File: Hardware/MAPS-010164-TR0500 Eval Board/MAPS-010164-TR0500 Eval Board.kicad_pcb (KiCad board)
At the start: 2 copper layers, 48.5 x 38.8 mm, 23 parts, among them IC1 MAPS-010164-TR0500, J1 Conn_Coaxial, J2 Conn_Coaxial, J3 Conn_02x02_Top_Bottom, J4 Conn_02x02_Top_Bottom, J5 Conn_02x04_Top_Bottom, J6 Conn_Coaxial, J7 Conn_Coaxial, J8 Conn_02x02_Top_Bottom

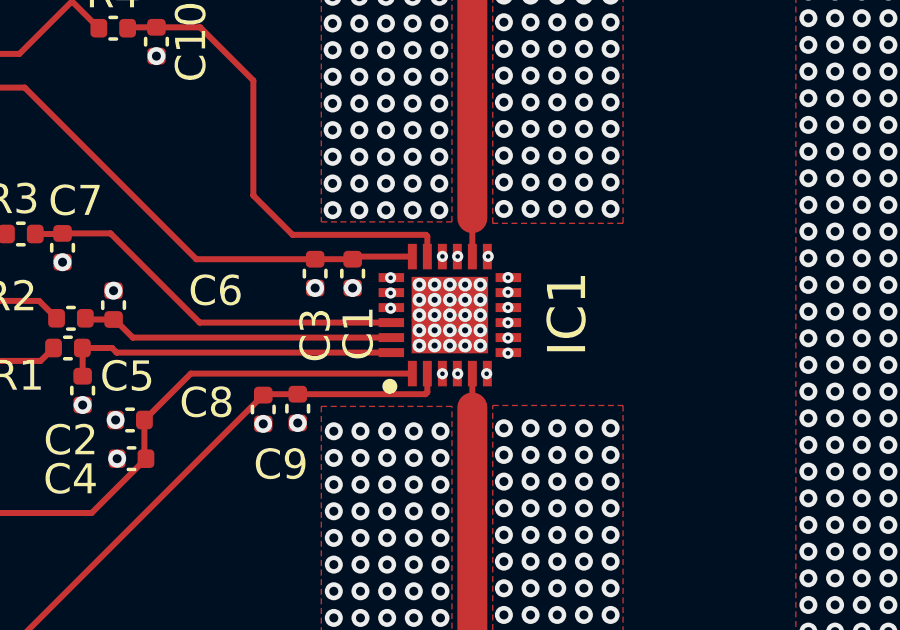
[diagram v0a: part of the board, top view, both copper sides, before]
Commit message: Fixed JLCPCB Errors
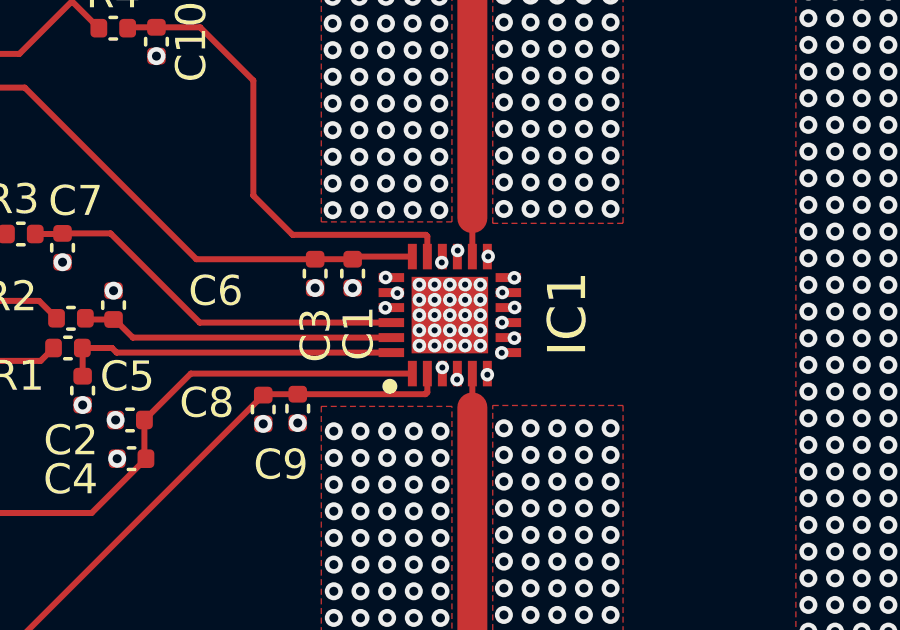
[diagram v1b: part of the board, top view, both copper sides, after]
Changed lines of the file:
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@@
 			(plot_on_all_layers_selection 0x00000000_00000000_00000000_00000000)
 			(disableapertmacros no)
-			(usegerberextensions no)
+			(usegerberextensions yes)
 			(usegerberattributes yes)
 			(usegerberadvancedattributes yes)
@@
 			(sketchdnponfab yes)
 			(crossoutdnponfab yes)
-			(subtractmaskfromsilk no)
+			(subtractmaskfromsilk yes)
 			(outputformat 1)
 			(mirror no)
-			(drillshape 1)
+			(drillshape 0)
 			(scaleselection 1)
-			(outputdirectory "")
+			(outputdirectory "MAPS-010164-TR500-EVAL-GRB/")
 		)
 	)
@@
 	(via
 		(at 106.5276 58.8772)
-		(size 0.375)
-		(drill 0.15)
+		(size 0.45)
+		(drill 0.2)
 		(layers "F.Cu" "B.Cu")
 		(net 1)
@@
 	)
 	(via
+		(at 103.11 59.58)
+		(size 0.45)
+		(drill 0.2)
+		(layers "F.Cu" "B.Cu")
+		(net 1)
+	)
+	(via
 		(at 117.202 59.8265)
 		(size 0.6)
@@
 	)
 	(via
+		(at 105.49 62.98)
+		(size 0.45)
+		(drill 0.2)
+		(layers "F.Cu" "B.Cu")
+		(net 1)
+	)
+	(via
 		(at 101.74 46.8225)
 		(size 0.6)
@@
 	)
 	(via
-		(at 107.188 61.087)
-		(size 0.375)
-		(drill 0.15)
-		(layers "F.Cu" "B.Cu")
-		(net 1)
-	)
-	(via
 		(at 119.869 48.2695)
 		(size 0.6)
@@
 	)
 	(via
+		(at 103.5 60.1)
+		(size 0.45)
+		(drill 0.2)
+		(layers "F.Cu" "B.Cu")
+		(net 1)
+	)
+	(via
 		(at 122.874 61.5)
 		(size 0.6)
@@
 	)
 	(via
-		(at 105.5116 62.7888)
-		(size 0.375)
-		(drill 0.15)
-		(layers "F.Cu" "B.Cu")
-		(net 1)
-	)
-	(via
 		(at 118.091 49.1585)
 		(size 0.6)
@@
 	)
 	(via
+		(at 106.5 62.82)
+		(size 0.45)
+		(drill 0.2)
+		(layers "F.Cu" "B.Cu")
+		(net 1)
+	)
+	(via
 		(at 104.01 51.112)
 		(size 0.6)
@@
 	)
 	(via
-		(at 103.2764 59.5884)
-		(size 0.375)
-		(drill 0.15)
-		(layers "F.Cu" "B.Cu")
-		(net 1)
-	)
-	(via
 		(at 107.052 72.606)
 		(size 0.6)
@@
 	)
 	(via
+		(at 105 62.58)
+		(size 0.45)
+		(drill 0.2)
+		(layers "F.Cu" "B.Cu")
+		(net 1)
+	)
+	(via
 		(at 118.091 52.7145)
 		(size 0.6)
@@
 	)
 	(via
+		(at 104.98 59.08)
+		(size 0.45)
+		(drill 0.2)
+		(layers "F.Cu" "B.Cu")
+		(net 1)
+	)
+	(via
 		(at 104.01 57.335)
 		(size 0.6)
@@
 	)
 	(via
-		(at 107.188 61.595)
-		(size 0.375)
-		(drill 0.15)
-		(layers "F.Cu" "B.Cu")
-		(net 1)
-	)
-	(via
 		(at 107.941 66.383)
 		(size 0.6)
@@
 	)
 	(via
-		(at 105.0036 62.7888)
-		(size 0.375)
-		(drill 0.15)
-		(layers "F.Cu" "B.Cu")
-		(net 1)
-	)
-	(via
 		(at 126.43 62.389)
 		(size 0.6)
@@
 	)
 	(via
-		(at 103.2764 60.6044)
-		(size 0.375)
-		(drill 0.15)
-		(layers "F.Cu" "B.Cu")
-		(net 1)
-	)
-	(via
 		(at 109.719 67.272)
 		(size 0.6)
@@
 	)
 	(via
+		(at 107.41 60.58)
+		(size 0.45)
+		(drill 0.2)
+		(layers "F.Cu" "B.Cu")
+		(net 1)
+	)
+	(via
 		(at 100.76 59.9302)
 		(size 0.6)
@@
 	)
 	(via
-		(at 103.2764 60.0964)
-		(size 0.375)
-		(drill 0.15)
-		(layers "F.Cu" "B.Cu")
-		(net 1)
-	)
-	(via
 		(at 101.382 65.594)
 		(size 0.6)
@@
 	)
 	(via
+		(at 105.51 58.68)
+		(size 0.45)
+		(drill 0.2)
+		(layers "F.Cu" "B.Cu")
+		(net 1)
+	)
+	(via
 		(at 101.74 75.48)
 		(size 0.6)
@@
 	)
 	(via
-		(at 107.188 60.579)
-		(size 0.375)
-		(drill 0.15)
-		(layers "F.Cu" "B.Cu")
-		(net 1)
-	)
-	(via
 		(at 119.869 67.8275)
 		(size 0.6)
@@
 	)
 	(via
-		(at 107.188 62.103)
-		(size 0.375)
-		(drill 0.15)
-		(layers "F.Cu" "B.Cu")
-		(net 1)
-	)
-	(via
 		(at 126.08 44.8025)
 		(size 0.6)
@@
 	)
 	(via
-		(at 107.188 60.071)
-		(size 0.375)
-		(drill 0.15)
-		(layers "F.Cu" "B.Cu")
-		(net 1)
-	)
-	(via
 		(at 104.938 67.372)
 		(size 0.6)
@@
 	)
 	(via
-		(at 107.19 59.583)
-		(size 0.375)
-		(drill 0.15)
-		(layers "F.Cu" "B.Cu")
-		(net 1)
-	)
-	(via
 		(at 107.941 48.405)
 		(size 0.6)
@@
 	)
 	(via
+		(at 106.98 62.09)
+		(size 0.45)
+		(drill 0.2)
+		(layers "F.Cu" "B.Cu")
+		(net 1)
+	)
+	(via
+		(at 107 60.08)
+		(size 0.45)
+		(drill 0.2)
+		(layers "F.Cu" "B.Cu")
+		(net 1)
+	)
+	(via
 		(at 119.869 50.0475)
 		(size 0.6)
@@
 	)
 	(via
+		(at 106.99 61.08)
+		(size 0.45)
+		(drill 0.2)
+		(layers "F.Cu" "B.Cu")
+		(net 1)
+	)
+	(via
 		(at 99.03 64.46)
 		(size 0.6)
@@
 	)
 	(via
-		(at 106.4768 62.7888)
-		(size 0.375)
-		(drill 0.15)
-		(layers "F.Cu" "B.Cu")
-		(net 1)
-	)
-	(via
 		(at 120.758 48.2695)
 		(size 0.6)
@@
 	)
 	(via
+		(at 107.4 59.59)
+		(size 0.45)
+		(drill 0.2)
+		(layers "F.Cu" "B.Cu")
+		(net 1)
+	)
+	(via
 		(at 119.869 64.2715)
 		(size 0.6)
@@
 	)
 	(via
-		(at 105.5116 58.8772)
-		(size 0.375)
-		(drill 0.15)
-		(layers "F.Cu" "B.Cu")
-		(net 1)
-	)
-	(via
 		(at 108.83 57.295)
 		(size 0.6)
@@
 	)
 	(via
-		(at 105.0036 58.8772)
-		(size 0.375)
-		(drill 0.15)
-		(layers "F.Cu" "B.Cu")
-		(net 1)
-	)
-	(via
 		(at 110.24 45.8225)
 		(size 0.6)
@@
 	)
 	(via
+		(at 103.1 60.59)
+		(size 0.45)
+		(drill 0.2)
+		(layers "F.Cu" "B.Cu")
+		(net 1)
+	)
+	(via
 		(at 105.25 59.817)
 		(size 0.4572)
@@
 		(layers "F.Cu" "B.Cu")
 		(net 1)
+	)
+	(via
+		(at 107.4 61.6)
+		(size 0.45)
+		(drill 0.2)
+		(layers "F.Cu" "B.Cu")
+		(net 1)
